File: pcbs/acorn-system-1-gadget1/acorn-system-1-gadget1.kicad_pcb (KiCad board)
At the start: 2 copper layers, 3 parts, among them J2 DIN41612_02x32_AB_acorn-syste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

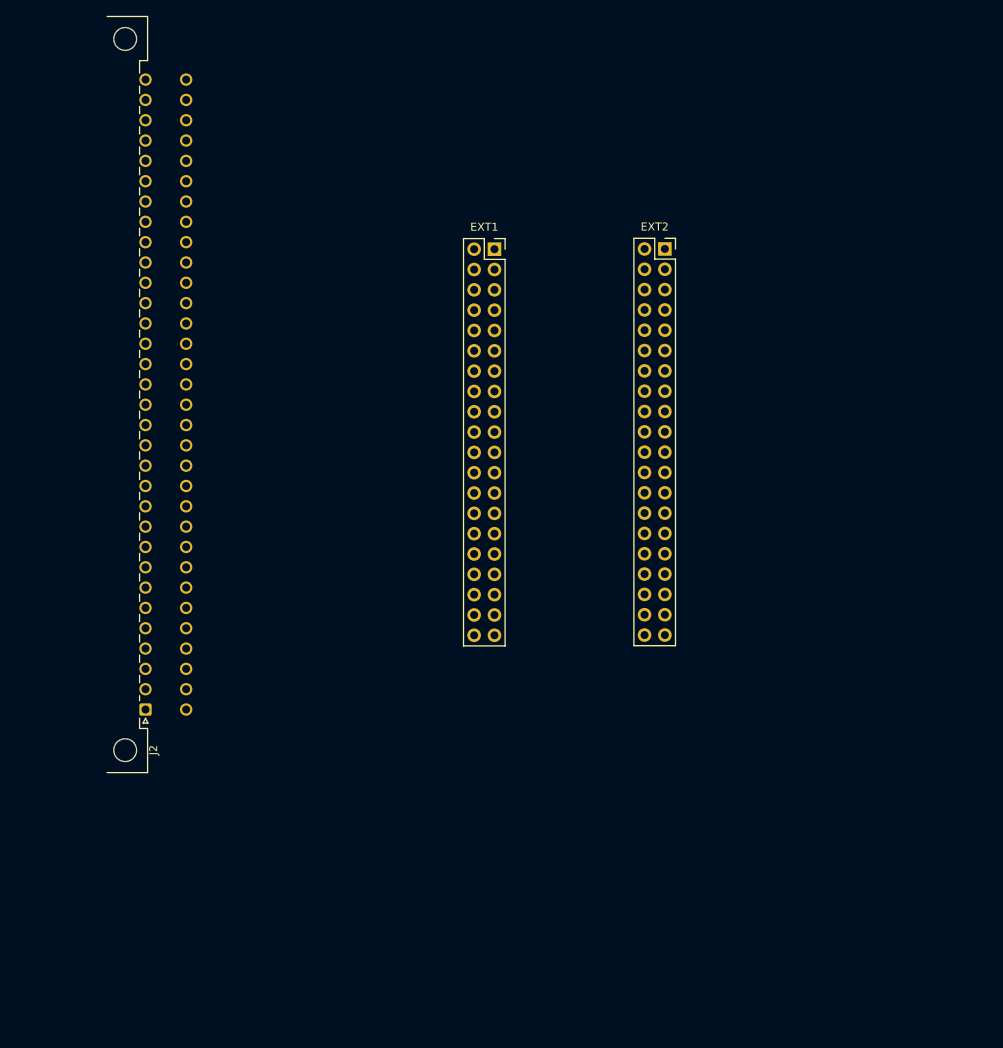
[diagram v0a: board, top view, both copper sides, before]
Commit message: "Update"
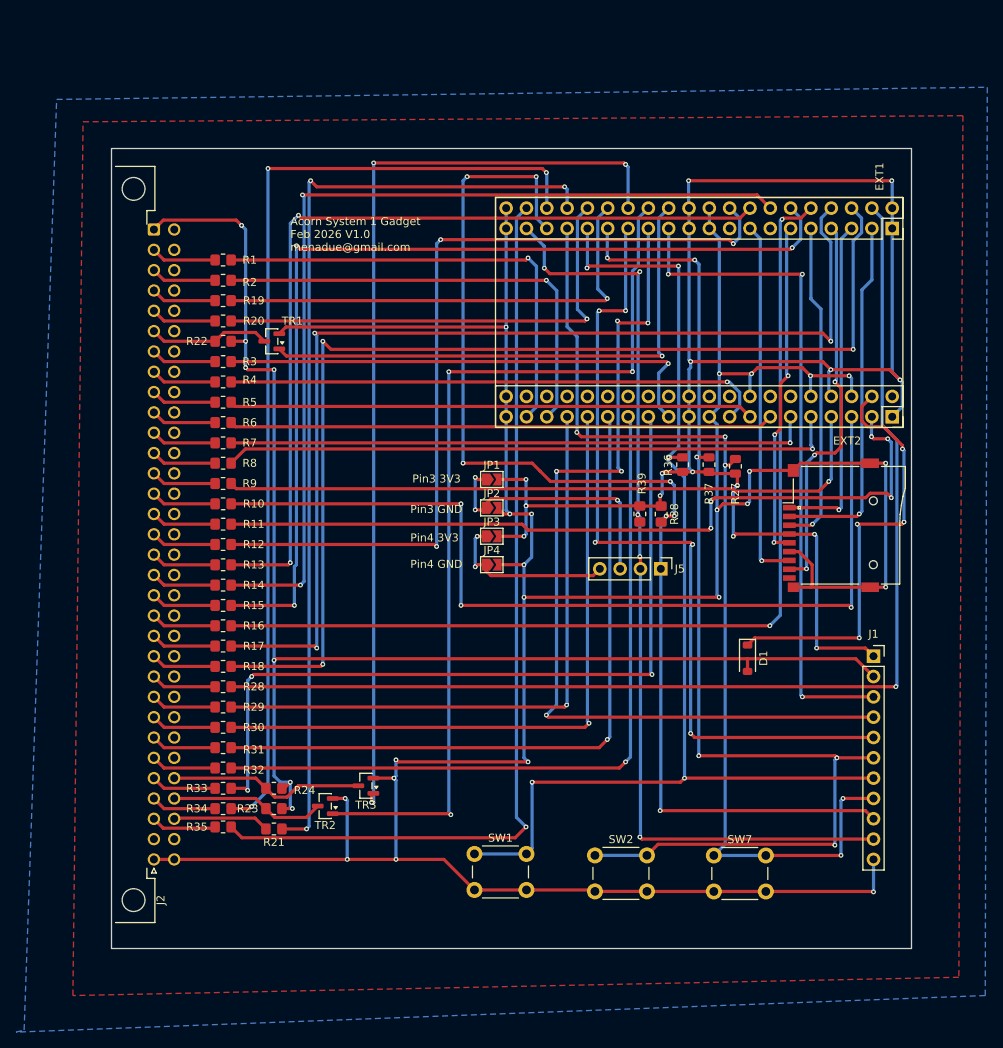
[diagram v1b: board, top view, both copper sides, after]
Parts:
- added D1: D_Schottky, Diode_SMD:D_SOD-123, F.Cu at (169.2, 118.6)
- added J1: Conn_01x11_Pin, Connector_PinSocket_2.54mm:PinSocket_1x11_P2.54mm_Vertical, F.Cu at (184.9, 118.3)
- added J5: Conn_01x04_Female, Connector_PinHeader_2.54mm:PinHeader_1x04_P2.54mm_Vertical, F.Cu at (158.4, 107.4)
- added JP1: Jumper_NO_Small, Jumper:SolderJumper-2_P1.3mm_Open_TrianglePad1.0x1.5mm, F.Cu at (137.2, 96.2)
- added JP2: Jumper_NO_Small, Jumper:SolderJumper-2_P1.3mm_Open_TrianglePad1.0x1.5mm, F.Cu at (137.2, 99.8)
- added JP3: Jumper_NO_Small, Jumper:SolderJumper-2_P1.3mm_Open_TrianglePad1.0x1.5mm, F.Cu at (137.2, 103.3)
- added JP4: Jumper_NO_Small, Jumper:SolderJumper-2_P1.3mm_Open_TrianglePad1.0x1.5mm, F.Cu at (137.2, 106.9)
- added R1: 1k, Resistor_SMD:R_0805_2012Metric_Pad1.20x1.40mm_HandSolder, F.Cu at (103.7, 68.8)
- added R10: 1k, Resistor_SMD:R_0805_2012Metric_Pad1.20x1.40mm_HandSolder, F.Cu at (103.7, 99.3)
- added R11: 1k, Resistor_SMD:R_0805_2012Metric_Pad1.20x1.40mm_HandSolder, F.Cu at (103.7, 101.8)
- added R12: 1k, Resistor_SMD:R_0805_2012Metric_Pad1.20x1.40mm_HandSolder, F.Cu at (103.7, 104.4)
- added R13: 1k, Resistor_SMD:R_0805_2012Metric_Pad1.20x1.40mm_HandSolder, F.Cu at (103.7, 106.9)
- added R14: 1k, Resistor_SMD:R_0805_2012Metric_Pad1.20x1.40mm_HandSolder, F.Cu at (103.7, 109.5)
- added R15: 1k, Resistor_SMD:R_0805_2012Metric_Pad1.20x1.40mm_HandSolder, F.Cu at (103.7, 112.0)
- added R16: 1k, Resistor_SMD:R_0805_2012Metric_Pad1.20x1.40mm_HandSolder, F.Cu at (103.7, 114.5)
- added R17: 1k, Resistor_SMD:R_0805_2012Metric_Pad1.20x1.40mm_HandSolder, F.Cu at (103.7, 117.1)
- added R18: 1k, Resistor_SMD:R_0805_2012Metric_Pad1.20x1.40mm_HandSolder, F.Cu at (103.7, 119.6)
- added R19: 1k, Resistor_SMD:R_0805_2012Metric_Pad1.20x1.40mm_HandSolder, F.Cu at (103.7, 73.9)
- added R2: 1k, Resistor_SMD:R_0805_2012Metric_Pad1.20x1.40mm_HandSolder, F.Cu at (103.7, 71.3)
- added R20: 1k, Resistor_SMD:R_0805_2012Metric_Pad1.20x1.40mm_HandSolder, F.Cu at (103.7, 76.4)
- added R21: 1k, Resistor_SMD:R_0805_2012Metric_Pad1.20x1.40mm_HandSolder, F.Cu at (110.0, 139.9)
- added R22: 4k7, Resistor_SMD:R_0805_2012Metric_Pad1.20x1.40mm_HandSolder, F.Cu at (103.7, 79.0)
- added R23: 4k7, Resistor_SMD:R_0805_2012Metric_Pad1.20x1.40mm_HandSolder, F.Cu at (110.0, 137.4)
- added R24: 4k7, Resistor_SMD:R_0805_2012Metric_Pad1.20x1.40mm_HandSolder, F.Cu at (110.0, 134.8)
- added R27: 10k, Resistor_SMD:R_0805_2012Metric, F.Cu at (167.7, 94.6)
- added R28: 1k, Resistor_SMD:R_0805_2012Metric_Pad1.20x1.40mm_HandSolder, F.Cu at (103.7, 122.2)
- added R29: 1k, Resistor_SMD:R_0805_2012Metric_Pad1.20x1.40mm_HandSolder, F.Cu at (103.7, 124.7)
- added R3: 1k, Resistor_SMD:R_0805_2012Metric_Pad1.20x1.40mm_HandSolder, F.Cu at (103.7, 81.5)
- added R30: 1k, Resistor_SMD:R_0805_2012Metric_Pad1.20x1.40mm_HandSolder, F.Cu at (103.7, 127.2)
- added R31: 1k, Resistor_SMD:R_0805_2012Metric_Pad1.20x1.40mm_HandSolder, F.Cu at (103.7, 129.8)
- added R32: 1k, Resistor_SMD:R_0805_2012Metric_Pad1.20x1.40mm_HandSolder, F.Cu at (103.7, 132.3)
- added R33: 1k, Resistor_SMD:R_0805_2012Metric_Pad1.20x1.40mm_HandSolder, F.Cu at (103.7, 134.8)
- added R34: 1k, Resistor_SMD:R_0805_2012Metric_Pad1.20x1.40mm_HandSolder, F.Cu at (103.7, 137.4)
- added R35: 1k, Resistor_SMD:R_0805_2012Metric_Pad1.20x1.40mm_HandSolder, F.Cu at (103.7, 139.7)
- added R36: 10k, Resistor_SMD:R_0805_2012Metric, F.Cu at (161.1, 94.4)
- added R37: 10k, Resistor_SMD:R_0805_2012Metric, F.Cu at (164.4, 94.4)
- added R38: 4k7, Resistor_SMD:R_0805_2012Metric_Pad1.20x1.40mm_HandSolder, F.Cu at (158.4, 100.6)
- added R39: 4k7, Resistor_SMD:R_0805_2012Metric_Pad1.20x1.40mm_HandSolder, F.Cu at (155.7, 100.6)
- added R4: 1k, Resistor_SMD:R_0805_2012Metric_Pad1.20x1.40mm_HandSolder, F.Cu at (103.7, 84.0)
- added R5: 1k, Resistor_SMD:R_0805_2012Metric_Pad1.20x1.40mm_HandSolder, F.Cu at (103.7, 86.6)
- added R6: 1k, Resistor_SMD:R_0805_2012Metric_Pad1.20x1.40mm_HandSolder, F.Cu at (103.7, 89.1)
- added R7: 1k, Resistor_SMD:R_0805_2012Metric_Pad1.20x1.40mm_HandSolder, F.Cu at (103.7, 91.7)
- added R8: 1k, Resistor_SMD:R_0805_2012Metric_Pad1.20x1.40mm_HandSolder, F.Cu at (103.7, 94.2)
- added R9: 1k, Resistor_SMD:R_0805_2012Metric_Pad1.20x1.40mm_HandSolder, F.Cu at (103.7, 96.8)
- added SW1: A, Button_Switch_THT:SW_PUSH_6mm, F.Cu at (135.1, 143.1)
- added SW2: A, Button_Switch_THT:SW_PUSH_6mm, F.Cu at (150.1, 143.2)
- added SW7: A, Button_Switch_THT:SW_PUSH_6mm, F.Cu at (165.0, 143.2)
- added TR1: Si2302CDS NCH, Package_TO_SOT_SMD:SOT-23, F.Cu at (109.7, 79.0)
- added TR2: Si2302CDS NCH, Package_TO_SOT_SMD:SOT-23, F.Cu at (116.4, 137.1)
- added TR3: Si2302CDS NCH, Package_TO_SOT_SMD:SOT-23, F.Cu at (121.5, 134.5)
- added XS1: 502p_SD_ebay-uSD-push_push_SMD, ajm-acorn:Conn_uSDcard, F.Cu at (184.9, 102.0)
- J2: footprint Connector_DIN:DIN41612_R_2x32_Female_Horizontal_THT -> ajm-acorn:DIN41612_Q_2x32_Female_Horizontal_THT
- moved EXT1 49.8 mm to (187.3, 64.9), turned to -90 degrees
- moved EXT2 35.3 mm to (187.3, 88.4), turned to -90 degrees
- moved J2 18.8 mm to (95.0, 143.7)
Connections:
- net /PICO-XL/3V3_EN renamed /3V3_EN
- net /PICO-XL/ADC_VREF renamed /ADC_VREF
- net /PICO-XL/BOOTSEL# renamed /BOOTSEL#
- net /PICO-XL/QSPI_CLK renamed /QSPI_CLK
- net /PICO-XL/QSPI_CSn renamed /QSPI_CSn
- net /PICO-XL/QSPI_SD0 renamed /QSPI_SD0
- net /PICO-XL/QSPI_SD1 renamed /QSPI_SD1
- net /PICO-XL/QSPI_SD2 renamed /QSPI_SD2
- net /PICO-XL/QSPI_SD3 renamed /QSPI_SD3
- net /PICO-XL/RUN renamed /RUN
- net /PICO-XL/SWCLK renamed /SWCLK
- net /PICO-XL/SWDIO renamed /SWDIO
- net GPIO23 renamed /GPIO23
- EXT1 pad 11: GPIO20 -> SD_CLK
- EXT1 pad 15: GPIO22 -> MISO_DO
- EXT1 pad 24: GPIO8 -> NRST_DRV
- EXT1 pad 26: GPIO9 -> NMI_DRV
- EXT1 pad 28: GPIO10 -> IRQ_DRV
- EXT1 pad 29: GPIO27 -> K3
- EXT1 pad 3: GPIO16 -> SD_SS
- EXT1 pad 30: GPIO11 -> NWDS
- EXT1 pad 31: GPIO28 -> K2
- EXT1 pad 32: GPIO12 -> NRDS
- EXT1 pad 33: GPIO29 -> K1
- EXT1 pad 34: GPIO13 -> SYNC
- EXT1 pad 35: GPIO30 -> I2C_SDA
- EXT1 pad 36: GPIO14 -> PHI2
- EXT1 pad 37: GPIO31 -> I2C_SCL
- EXT1 pad 38: GPIO15 -> RW
- EXT1 pad 5: GPIO17 -> SD_DAT2
- EXT1 pad 7: GPIO18 -> SD_DAT1
- EXT1 pad 9: GPIO19 -> MOSI_DI
- J2 pad a1: unconnected-(J2-Pin_a1-Pada1) -> +5V
- J2 pad a10: GPIO37 -> Net-(J2-Pin_a10)
- J2 pad a11: GPIO36 -> Net-(J2-Pin_a11)
- J2 pad a12: GPIO35 -> Net-(J2-Pin_a12)
- J2 pad a13: GPIO34 -> Net-(J2-Pin_a13)
- J2 pad a14: GPIO33 -> Net-(J2-Pin_a14)
- J2 pad a15: GPIO32 -> Net-(J2-Pin_a15)
- J2 pad a16: GPIO7 -> Net-(J2-Pin_a16)
- J2 pad a17: GPIO6 -> Net-(J2-Pin_a17)
- J2 pad a18: GPIO5 -> Net-(J2-Pin_a18)
- J2 pad a19: GPIO4 -> Net-(J2-Pin_a19)
- J2 pad a2: GPIO47 -> Net-(J2-Pin_a2)
- J2 pad a20: GPIO3 -> Net-(J2-Pin_a20)
- J2 pad a21: GPIO2 -> Net-(J2-Pin_a21)
- J2 pad a22: GPIO1 -> Net-(J2-Pin_a22)
- J2 pad a23: GPIO0 -> Net-(J2-Pin_a23)
- J2 pad a24: GPIO45 -> Net-(J2-Pin_a24)
- J2 pad a25: GPIO44 -> Net-(J2-Pin_a25)
- J2 pad a26: GPIO43 -> Net-(J2-Pin_a26)
- J2 pad a27: GPIO42 -> Net-(J2-Pin_a27)
- J2 pad a28: GPIO41 -> Net-(J2-Pin_a28)
- J2 pad a29: unconnected-(J2-Pin_a29-Pada29) -> Net-(J2-Pin_a29)
- J2 pad a3: GPIO46 -> Net-(J2-Pin_a3)
- J2 pad a30: unconnected-(J2-Pin_a30-Pada30) -> Net-(J2-Pin_a30)
- J2 pad a32: unconnected-(J2-Pin_a32-Pada32) -> GND
- J2 pad a4: unconnected-(J2-Pin_a4-Pada4) -> Net-(J2-Pin_a4)
- J2 pad a5: unconnected-(J2-Pin_a5-Pada5) -> Net-(J2-Pin_a5)
- J2 pad a6: unconnected-(J2-Pin_a6-Pada6) -> NRST
- J2 pad a7: GPIO40 -> Net-(J2-Pin_a7)
- J2 pad a8: GPIO39 -> Net-(J2-Pin_a8)
- J2 pad a9: GPIO38 -> Net-(J2-Pin_a9)
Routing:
- net GND: track 0.00 -> 402.4 mm, vias 0 -> 22
- net +3.3V: track 0.00 -> 208.9 mm, vias 0 -> 15
- net +5V: track 0.00 -> 171.9 mm, vias 0 -> 7
- net I2C_SDA: track 0.00 -> 149.3 mm, vias 0 -> 7
- net GPIO0: track 0.00 -> 144.3 mm, vias 0 -> 1
- net K2: track 0.00 -> 142.4 mm, vias 0 -> 5
- net K3: track 0.00 -> 142.3 mm, vias 0 -> 6
- net GPIO1: track 0.00 -> 137.3 mm, vias 0 -> 3
- net GPIO2: track 0.00 -> 132.9 mm, vias 0 -> 3
- net K1: track 0.00 -> 126.3 mm, vias 0 -> 5
- net GPIO3: track 0.00 -> 123.0 mm, vias 0 -> 2
- net PHI2: track 0.00 -> 122.8 mm, vias 0 -> 3
- net GPIO4: track 0.00 -> 121.1 mm, vias 0 -> 3
- net I2C_SCL: track 0.00 -> 119.5 mm, vias 0 -> 5
- net SYNC: track 0.00 -> 119.2 mm, vias 0 -> 3
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- added copper zone on B.Cu, net +3.3V
- added copper zone on F.Cu, net GND
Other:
- board outline added: 100 x 100 mm
- board text added: "Acorn System 1 Gadget Feb 2026 V1.0 menadue@gmail.com"
- board text added: "Pin3 3V3"
- board text added: "Pin3 GND"
- board text added: "Pin4 3V3"
- board text added: "Pin4 GND"
